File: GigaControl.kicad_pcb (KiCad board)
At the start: 6 copper layers, 40 x 20 mm, 49 parts, among them U1 LSM6DS3TR-C, U2 SIT3051, U3 REF3033AIDBZR, U4 PESD4USB5U-TTSX, U5 PESD4USB5U-TTSX, U6 STM32F405RGT6, U7 PESD4USB5U-TTSX, U8 PESD4USB5U-TTSX, Y1 SX2M8.000M20F30TNN

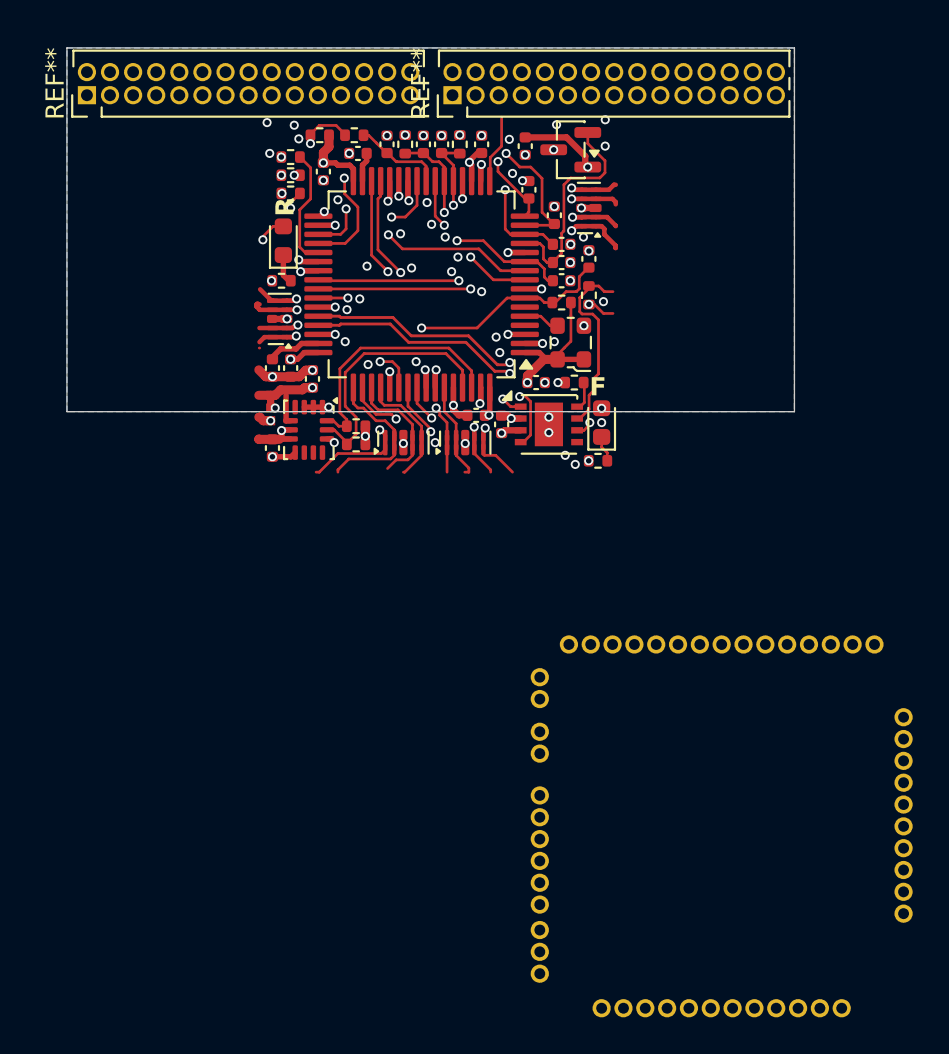
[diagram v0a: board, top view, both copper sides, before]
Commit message: initial
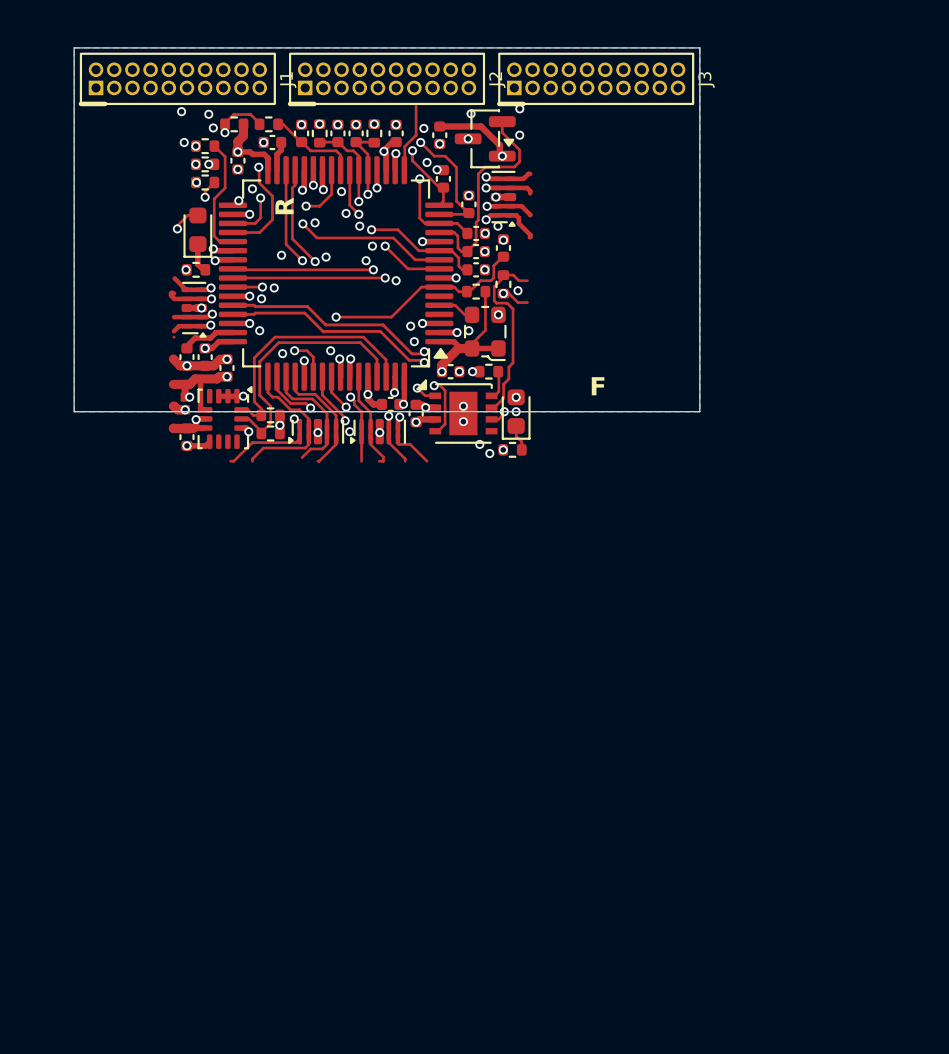
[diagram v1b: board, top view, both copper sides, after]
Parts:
- removed J4: ~, X3.0CH-Library:X3.0CH-Master
- removed REF** (x2): PinHeader_2x15_P1.27mm_Vertical, Connector_PinHeader_1.27mm:PinHeader_2x15_P1.27mm_Vertical
- added J1: Conn_02x10_Odd_Even, X3.0CH-Library:Hanxia_HX_PM1.0-2x10P_ZC, F.Cu at (138.6, 87.7)
- added J2: Conn_02x10_Odd_Even, X3.0CH-Library:Hanxia_HX_PM1.0-2x10P_ZC, F.Cu at (150.1, 87.7)
- added J3: Conn_02x10_Odd_Even, X3.0CH-Library:Hanxia_HX_PM1.0-2x10P_ZC, F.Cu at (161.6, 87.7)
- moved C27 4.74 mm to (159.1, 94.1)
- moved C3 4.74 mm to (156.2, 105.6)
- moved C47 4.74 mm to (158.1, 103.3)
- moved R3 4.74 mm to (160.2, 103.3)
- moved U5 4.74 mm to (154.2, 106.6)
- moved C16 4.74 mm to (143.6, 102.5)
- moved C18 4.74 mm to (155.1, 90.2)
- moved C2 4.74 mm to (143.6, 106.9)
- moved C20 4.74 mm to (144.6, 102.5)
- moved C28 4.74 mm to (157.7, 92.7)
- moved D1 4.74 mm to (144.2, 95.5)
- moved D2 4.74 mm to (161.7, 105.5)
- moved R1 4.74 mm to (148.2, 105.7)
- moved R11 4.74 mm to (144.1, 97.7)
- moved R13 4.74 mm to (146.2, 89.7)
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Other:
- board size 40 x 20 mm -> 34.4 x 20 mm

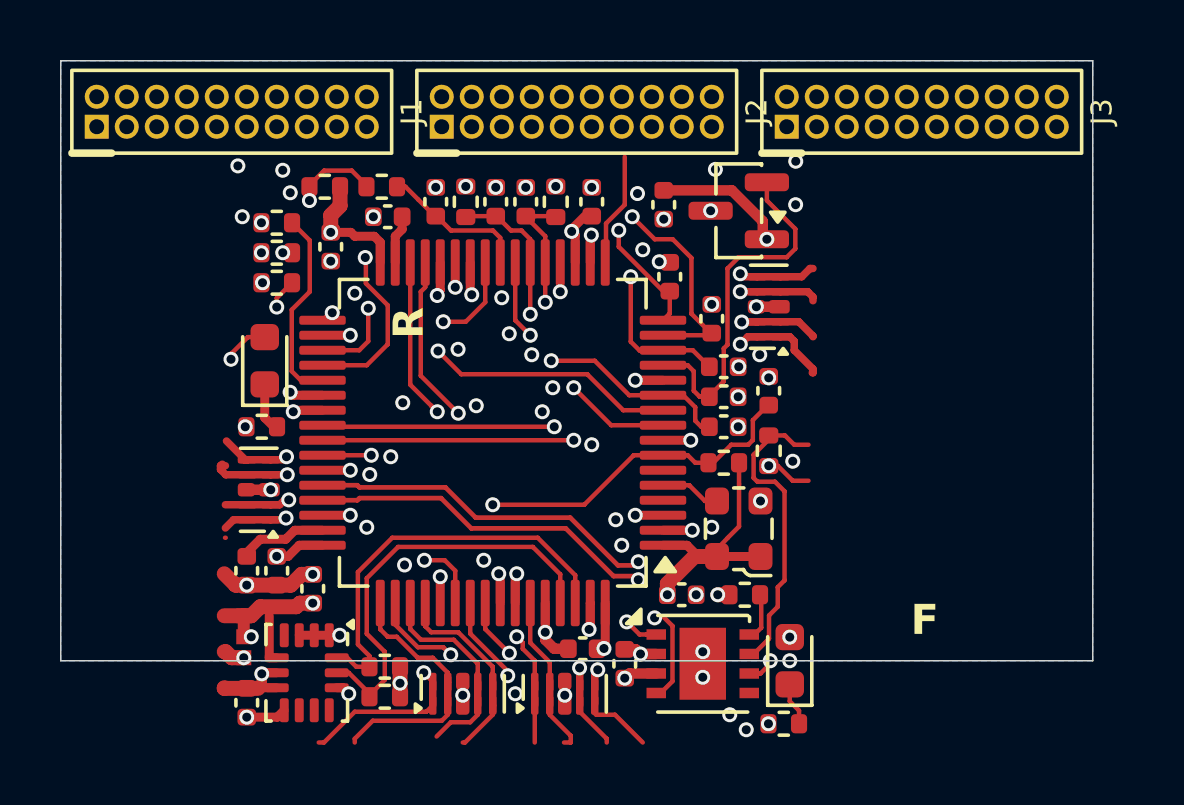
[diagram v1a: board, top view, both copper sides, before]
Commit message: initial
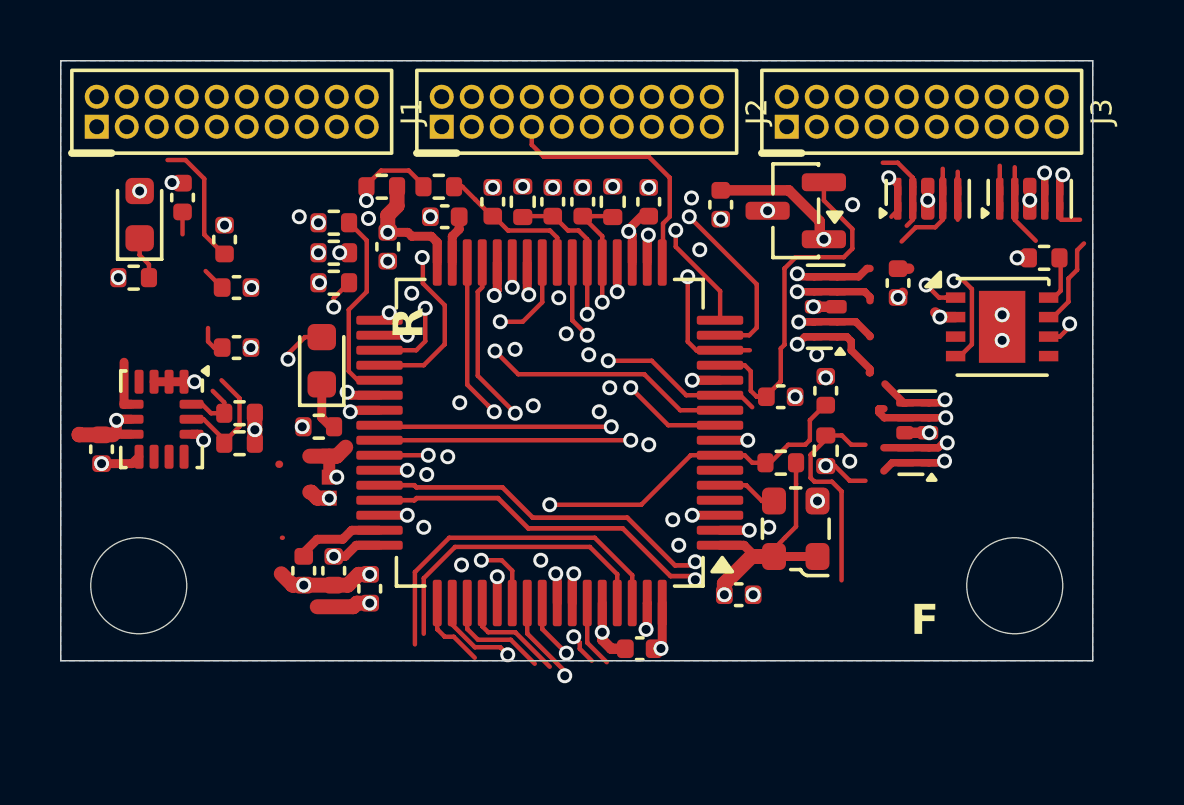
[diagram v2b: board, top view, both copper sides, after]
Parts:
- added H1: MountingHole_3.2mm_M3, MountingHole:MountingHole_3.2mm_M3, F.Cu at (140.0, 103.0)
- added H2: MountingHole_3.2mm_M3, MountingHole:MountingHole_3.2mm_M3, F.Cu at (169.2, 103.0)
- moved D2 26.3 mm to (140.0, 90.6)
- moved R12 26.3 mm to (139.8, 92.7)
- moved U5 22.6 mm to (169.7, 90.1)
- moved U7 22.6 mm to (166.3, 90.1)
- moved U8 22.0 mm to (165.9, 97.9)
- moved C26 16.5 mm to (143.3, 93.1)
- moved C30 16.5 mm to (143.3, 95.1)
- moved C27 16.5 mm to (142.9, 91.5)
- moved C28 16.5 mm to (141.5, 90.1)
- moved C3 15.6 mm to (165.3, 92.9)
- moved R3 15.0 mm to (170.2, 92.1)
- moved U2 15.0 mm to (168.8, 94.4)
- moved C2 9.74 mm to (138.8, 98.5)
- moved U1 9.74 mm to (140.8, 97.5)
- moved R1 9.74 mm to (143.4, 97.2)
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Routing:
- net +5V: track 39.5 -> 20.0 mm, vias 3 -> 2
- net SPI1-MOSI: track 13.1 -> 23.6 mm
- net VSENSE2: track 9.60 -> 18.4 mm
- net CURR1 FILTERED: track 11.1 -> 17.4 mm
- net VSENSE3: track 12.7 -> 18.9 mm
- net CURR3 FILTERED: track 15.8 -> 21.0 mm
- net H1: track 19.2 -> 24.2 mm
- net H3: track 13.1 -> 18.1 mm
- net L3: track 9.42 -> 14.4 mm
- net MOSTEMP1: track 3.79 -> 8.58 mm
- net MOSTEMP2: track 6.07 -> 10.8 mm
- net RESERVED2: track 9.56 -> 4.90 mm
- net RESERVED3: track 10.1 -> 5.59 mm
- net H2: track 13.2 -> 17.7 mm
- net MOSTEMP3: track 10.4 -> 14.5 mm
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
